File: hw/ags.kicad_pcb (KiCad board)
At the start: 4 copper layers, 0 parts

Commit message: Footprints created, starting layout
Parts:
- added C1: 22u, Capacitor_SMD:C_0603_1608Metric, F.Cu at (201.8, 34.2)
- added C10: 1u, Capacitor_SMD:C_0603_1608Metric, F.Cu at (232.0, 80.6)
- added C11: 2.7n, Capacitor_SMD:C_0603_1608Metric, F.Cu at (232.0, 83.1)
- added C12: 1u, Capacitor_SMD:C_0603_1608Metric, F.Cu at (211.8, 100.0)
- added C13: 1u, Capacitor_SMD:C_0603_1608Metric, F.Cu at (232.0, 61.1)
- added C14: 2.7n, Capacitor_SMD:C_0603_1608Metric, F.Cu at (232.0, 63.7)
- added C15: 2.7n, Capacitor_SMD:C_0603_1608Metric, F.Cu at (211.8, 102.5)
- added C16: 1u, Capacitor_SMD:C_0603_1608Metric, F.Cu at (211.8, 80.6)
- added C17: 2.7n, Capacitor_SMD:C_0603_1608Metric, F.Cu at (211.8, 83.1)
- added C18: 1u, Capacitor_SMD:C_0603_1608Metric, F.Cu at (211.8, 61.1)
- added C19: 2.7n, Capacitor_SMD:C_0603_1608Metric, F.Cu at (211.8, 63.7)
- added C2: 100n, Capacitor_SMD:C_0603_1608Metric, F.Cu at (201.8, 36.7)
- added C20: 1u, Capacitor_SMD:C_0603_1608Metric, F.Cu at (175.6, 92.9)
- added C21: 2.7n, Capacitor_SMD:C_0603_1608Metric, F.Cu at (175.6, 95.4)
- added C22: 1u, Capacitor_SMD:C_0603_1608Metric, F.Cu at (232.0, 100.0)
- added C23: 2.7n, Capacitor_SMD:C_0603_1608Metric, F.Cu at (232.0, 102.5)
- added C24: 100n, Capacitor_SMD:C_0603_1608Metric, F.Cu at (224.9, 39.2)
- added C3: 1u, Capacitor_SMD:C_0603_1608Metric, F.Cu at (201.8, 39.2)
- added C4: 1u, Capacitor_SMD:C_0603_1608Metric, F.Cu at (201.8, 41.7)
- added C5: 1u, Capacitor_SMD:C_0603_1608Metric, F.Cu at (155.3, 92.9)
- added C6: 4.7u, Capacitor_SMD:C_1210_3225Metric, F.Cu at (230.9, 54.6)
- added C7: 100n, Capacitor_SMD:C_0603_1608Metric, F.Cu at (224.9, 34.2)
- added C8: 22u, Capacitor_SMD:C_0603_1608Metric, F.Cu at (224.9, 36.7)
- added C9: 2.7n, Capacitor_SMD:C_0603_1608Metric, F.Cu at (155.3, 95.4)
- added D1: B38G3RGB-10D0003H2U1930, qmi_footprints:B38G3RGB-10D0003H2U1930, F.Cu at (201.1, 50.2)
- added D10: SMAJ60CA, Diode_SMD:D_SMA, F.Cu at (217.9, 113.8)
- added D11: SM4007PL, Diode_SMD:D_SOD-123F, F.Cu at (225.3, 88.0)
- added D12: SMAJ60CA, Diode_SMD:D_SMA, F.Cu at (217.9, 94.4)
- added D13: SM4007PL, Diode_SMD:D_SOD-123F, F.Cu at (225.3, 68.6)
- added D14: SMAJ60CA, Diode_SMD:D_SMA, F.Cu at (217.9, 75.0)
- added D15: SM4007PL, Diode_SMD:D_SOD-123F, F.Cu at (189.1, 100.3)
- added D16: SMAJ60CA, Diode_SMD:D_SMA, F.Cu at (181.6, 106.8)
- added D17: SM4007PL, Diode_SMD:D_SOD-123F, F.Cu at (245.6, 107.4)
- added D18: SMAJ60CA, Diode_SMD:D_SMA, F.Cu at (238.1, 113.8)
- added D19: SM4007PL, Diode_SMD:D_SOD-123F, F.Cu at (245.6, 71.9)
- added D2: SMAJ60CA, Diode_SMD:D_SMA, F.Cu at (238.1, 75.0)
- added D20: SM4007PL, Diode_SMD:D_SOD-123F, F.Cu at (168.8, 103.7)
- added D21: SM4007PL, Diode_SMD:D_SOD-123F, F.Cu at (245.6, 91.3)
- added D22: SM4007PL, Diode_SMD:D_SOD-123F, F.Cu at (225.3, 110.8)
- added D23: SM4007PL, Diode_SMD:D_SOD-123F, F.Cu at (225.3, 91.3)
- added D24: SM4007PL, Diode_SMD:D_SOD-123F, F.Cu at (225.3, 71.9)
- added D25: SM4007PL, Diode_SMD:D_SOD-123F, F.Cu at (189.1, 103.7)
- added D26: SM4007PL, Diode_SMD:D_SOD-123F, F.Cu at (245.6, 110.8)
- added D27: SM4007PL, Diode_SMD:D_SOD-123F, F.Cu at (229.7, 42.7)
- added D3: SM4007PL, Diode_SMD:D_SOD-123F, F.Cu at (245.6, 68.6)
- added D4: SMAJ60CA, Diode_SMD:D_SMA, F.Cu at (213.8, 55.6)
- added D5: SM4007PL, Diode_SMD:D_SOD-123F, F.Cu at (168.8, 100.3)
- added D6: SMAJ60CA, Diode_SMD:D_SMA, F.Cu at (161.4, 106.8)
- added D7: SM4007PL, Diode_SMD:D_SOD-123F, F.Cu at (245.6, 88.0)
- added D8: SM4007PL, Diode_SMD:D_SOD-123F, F.Cu at (225.3, 107.4)
- added D9: SMAJ60CA, Diode_SMD:D_SMA, F.Cu at (238.1, 94.4)
- added F1: 0ZCF0075AF2C, Fuse:Fuse_2920_7451Metric, F.Cu at (228.0, 49.0)
- added F2: 0ZCF0075AF2C, Fuse:Fuse_2920_7451Metric, F.Cu at (239.2, 63.4)
- added F3: 0ZCF0075AF2C, Fuse:Fuse_2920_7451Metric, F.Cu at (162.4, 95.2)
- added F4: 0ZCF0075AF2C, Fuse:Fuse_2920_7451Metric, F.Cu at (239.2, 82.8)
- added F5: 0ZCF0075AF2C, Fuse:Fuse_2920_7451Metric, F.Cu at (218.9, 102.2)
- added F6: 0ZCF0075AF2C, Fuse:Fuse_2920_7451Metric, F.Cu at (218.9, 82.8)
- added F7: 0ZCF0075AF2C, Fuse:Fuse_2920_7451Metric, F.Cu at (218.9, 63.4)
- added F8: 0ZCF0075AF2C, Fuse:Fuse_2920_7451Metric, F.Cu at (182.7, 95.2)
- added F9: 0ZCF0075AF2C, Fuse:Fuse_2920_7451Metric, F.Cu at (239.2, 102.2)
- added J1: Screw_Terminal_01x08, qmi_footprints:QT08ASF83H0000G, F.Cu at (166.9, 132.4)
- added J9: Screw_Terminal_01x02, qmi_footprints:QT02ASF83H0000G, F.Cu at (121.9, 128.9)
- added L1: 22u HPC 6045NV-220M, qmi_footprints:HPC 6045NV-220M, F.Cu at (231.0, 37.0)
- added R1: 1k, Resistor_SMD:R_0603_1608Metric, F.Cu at (201.8, 44.2)
- added R10: 270, Resistor_SMD:R_0603_1608Metric, F.Cu at (211.8, 105.0)
- added R11: 270, Resistor_SMD:R_0603_1608Metric, F.Cu at (232.0, 66.2)
- added R12: 113k 1%, Resistor_SMD:R_0603_1608Metric, F.Cu at (211.8, 107.5)
- added R13: 113k 1%, Resistor_SMD:R_0603_1608Metric, F.Cu at (232.0, 68.7)
- added R14: 32k 1%, Resistor_SMD:R_0603_1608Metric, F.Cu at (224.9, 41.7)
- added R15: 5.90k 1%, Resistor_SMD:R_0603_1608Metric, F.Cu at (201.8, 46.7)
- added R16: 5.90k 1%, Resistor_SMD:R_0603_1608Metric, F.Cu at (211.8, 110.0)
- added R17: 100 ERJ-P06F1000V, Resistor_SMD:R_0805_2012Metric, F.Cu at (224.7, 113.9)
- added R18: 5.90k 1%, Resistor_SMD:R_0603_1608Metric, F.Cu at (232.0, 71.2)
- added R19: 5.90k 1%, Resistor_SMD:R_0603_1608Metric, F.Cu at (205.8, 34.2)
- added R2: 270, Resistor_SMD:R_0603_1608Metric, F.Cu at (155.3, 97.9)
- added R20: 100 ERJ-P06F1000V, Resistor_SMD:R_0805_2012Metric, F.Cu at (245.0, 75.1)
- added R21: 270, Resistor_SMD:R_0603_1608Metric, F.Cu at (211.8, 85.6)
- added R22: 113k 1%, Resistor_SMD:R_0603_1608Metric, F.Cu at (211.8, 88.1)
- added R23: 5.90k 1%, Resistor_SMD:R_0603_1608Metric, F.Cu at (211.8, 90.6)
- added R24: 100 ERJ-P06F1000V, Resistor_SMD:R_0805_2012Metric, F.Cu at (224.7, 94.5)
- added R25: 270, Resistor_SMD:R_0603_1608Metric, F.Cu at (211.8, 66.2)
- added R26: 113k 1%, Resistor_SMD:R_0603_1608Metric, F.Cu at (211.8, 68.7)
- added R27: 5.90k 1%, Resistor_SMD:R_0603_1608Metric, F.Cu at (211.8, 71.2)
- added R28: 100 ERJ-P06F1000V, Resistor_SMD:R_0805_2012Metric, F.Cu at (224.7, 75.1)
- added R29: 270, Resistor_SMD:R_0603_1608Metric, F.Cu at (175.6, 97.9)
- added R3: 113k 1%, Resistor_SMD:R_0603_1608Metric, F.Cu at (155.3, 100.4)
- added R30: 113k 1%, Resistor_SMD:R_0603_1608Metric, F.Cu at (175.6, 100.4)
- added R31: 5.90k 1%, Resistor_SMD:R_0603_1608Metric, F.Cu at (175.6, 102.9)
- added R32: 100 ERJ-P06F1000V, Resistor_SMD:R_0805_2012Metric, F.Cu at (188.5, 106.8)
- added R33: 270, Resistor_SMD:R_0603_1608Metric, F.Cu at (232.0, 105.0)
- added R34: 113k 1%, Resistor_SMD:R_0603_1608Metric, F.Cu at (232.0, 107.5)
- added R35: 5.90k 1%, Resistor_SMD:R_0603_1608Metric, F.Cu at (232.0, 110.0)
- added R36: 100 ERJ-P06F1000V, Resistor_SMD:R_0805_2012Metric, F.Cu at (245.0, 113.9)
- added R37: 1k, Resistor_SMD:R_0603_1608Metric, F.Cu at (205.8, 36.7)
- added R38: 1k, Resistor_SMD:R_0603_1608Metric, F.Cu at (205.8, 39.2)
- added R39: 1k, Resistor_SMD:R_0603_1608Metric, F.Cu at (205.8, 41.7)
- added R4: 5.90k 1%, Resistor_SMD:R_0603_1608Metric, F.Cu at (155.3, 102.9)
- added R40: 270, Resistor_SMD:R_0603_1608Metric, F.Cu at (205.8, 44.2)
- added R41: 100k 1%, Resistor_SMD:R_0603_1608Metric, F.Cu at (224.9, 44.2)
- added R5: 100 ERJ-P06F1000V, Resistor_SMD:R_0805_2012Metric, F.Cu at (168.3, 106.8)
- added R6: 270, Resistor_SMD:R_0603_1608Metric, F.Cu at (232.0, 85.6)
- added R7: 113k 1%, Resistor_SMD:R_0603_1608Metric, F.Cu at (232.0, 88.1)
- added R8: 5.90k 1%, Resistor_SMD:R_0603_1608Metric, F.Cu at (232.0, 90.6)
- added R9: 100 ERJ-P06F1000V, Resistor_SMD:R_0805_2012Metric, F.Cu at (245.0, 94.5)
- added SW1: PTS526SM15SMTR2 LFS, qmi_footprints:SON4_PTS526 SM15 SMTR2 LFS_CNK, F.Cu at (200.9, 72.8)
- added U1: GAQY212GSX, Package_SO:SO-4_4.4x4.3mm_P2.54mm, F.Cu at (161.7, 101.6)
- added U10: GAQY212GSX, Package_SO:SO-4_4.4x4.3mm_P2.54mm, F.Cu at (181.9, 101.6)
- added U11: GAQY212GSX, Package_SO:SO-4_4.4x4.3mm_P2.54mm, F.Cu at (238.4, 108.7)
- added U12: NV24C08DWVLT3G, Package_SO:SOIC-8_3.9x4.9mm_P1.27mm, F.Cu at (200.6, 79.7)
- added U2: GAQY212GSX, Package_SO:SO-4_4.4x4.3mm_P2.54mm, F.Cu at (238.4, 89.2)
- added U3: GAQY212GSX, Package_SO:SO-4_4.4x4.3mm_P2.54mm, F.Cu at (218.2, 108.7)
- added U4: LMR51610XDBVR, Package_TO_SOT_SMD:SOT-23-6, F.Cu at (225.5, 54.9)
- added U5: ESP32-S3-MINI-1, RF_Module:ESP32-S2-MINI-1, F.Cu at (150.2, 66.2)
- added U6: GAQY212GSX, Package_SO:SO-4_4.4x4.3mm_P2.54mm, F.Cu at (238.4, 69.8)
- added U7: GAQY212GSX, Package_SO:SO-4_4.4x4.3mm_P2.54mm, F.Cu at (218.2, 89.2)
- added U9: GAQY212GSX, Package_SO:SO-4_4.4x4.3mm_P2.54mm, F.Cu at (218.2, 69.8)

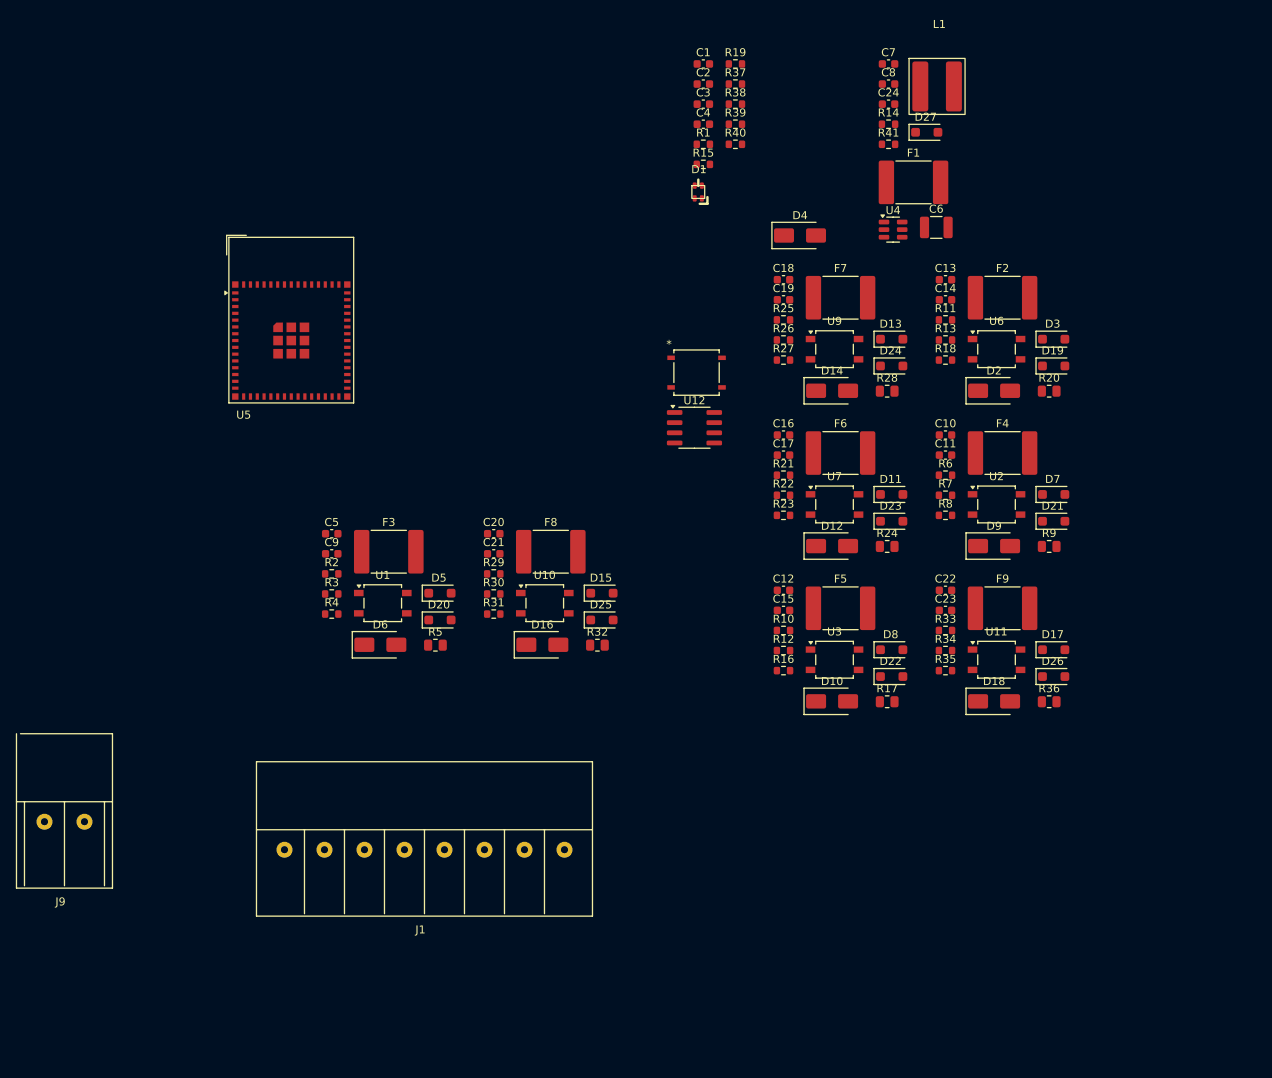
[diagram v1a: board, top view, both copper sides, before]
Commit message: Initial start to PCB
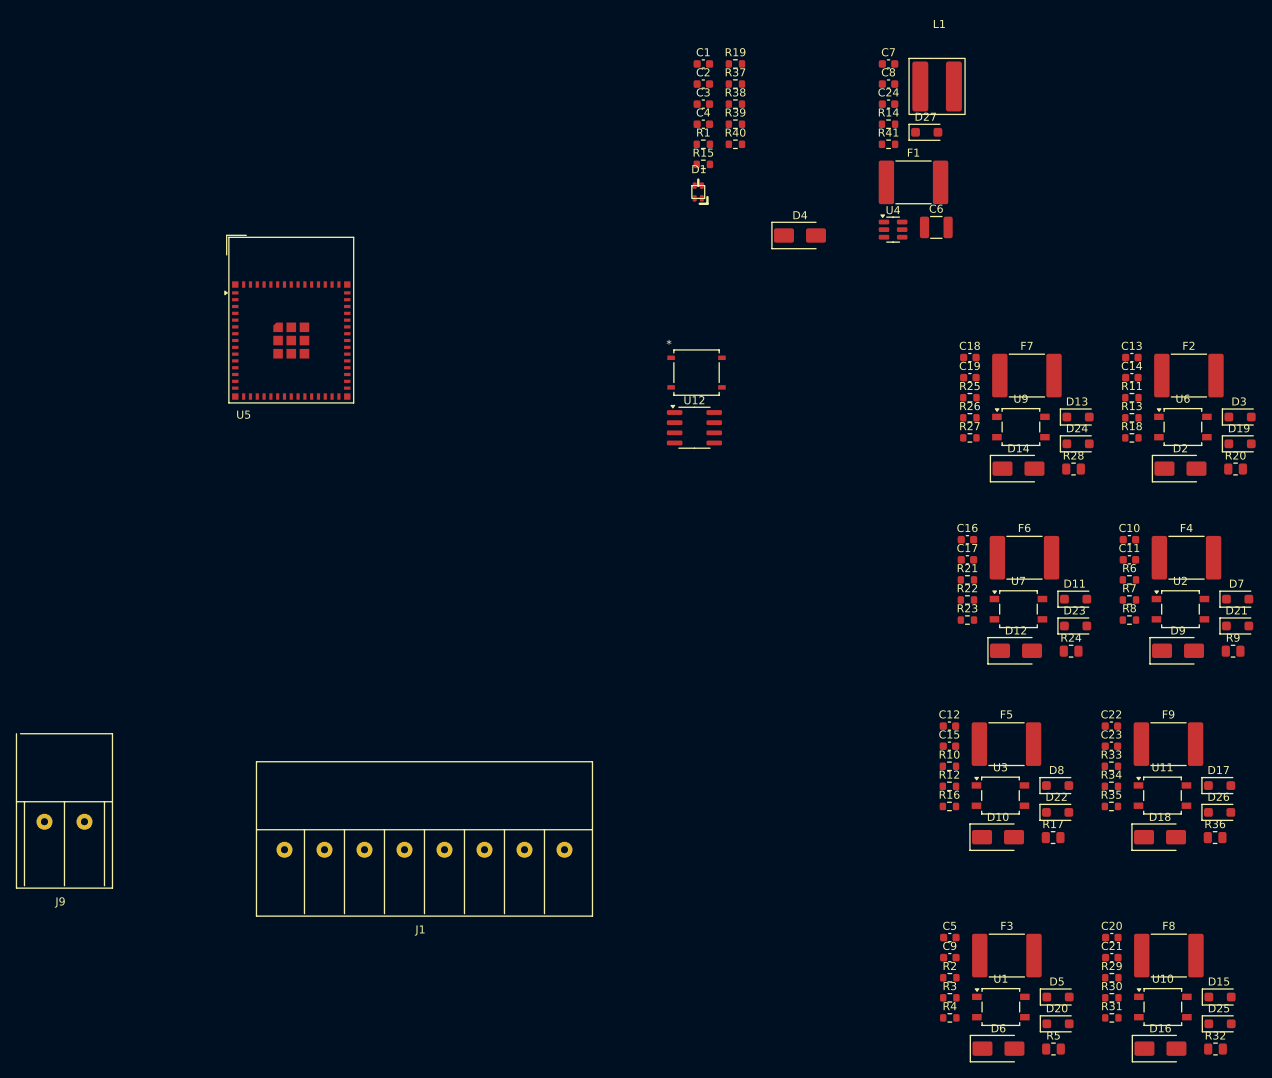
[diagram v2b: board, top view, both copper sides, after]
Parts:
- moved D6 92.3 mm to (238.6, 157.3)
- moved D5 92.3 mm to (246.1, 150.8)
- moved R2 92.3 mm to (232.6, 148.4)
- moved R29 92.3 mm to (252.8, 148.4)
- moved R5 92.3 mm to (245.5, 157.3)
- moved U1 92.3 mm to (238.9, 152.1)
- moved U10 92.3 mm to (259.2, 152.1)
- moved C20 92.3 mm to (252.8, 143.4)
- moved C21 92.3 mm to (252.8, 145.9)
- moved C5 92.3 mm to (232.6, 143.4)
- moved C9 92.3 mm to (232.6, 145.9)
- moved D16 92.3 mm to (258.9, 157.3)
- moved D20 92.3 mm to (246.1, 154.2)
- moved F3 92.3 mm to (239.7, 145.6)
- moved F8 92.3 mm to (259.9, 145.6)
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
